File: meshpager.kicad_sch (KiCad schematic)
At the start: 0 parts

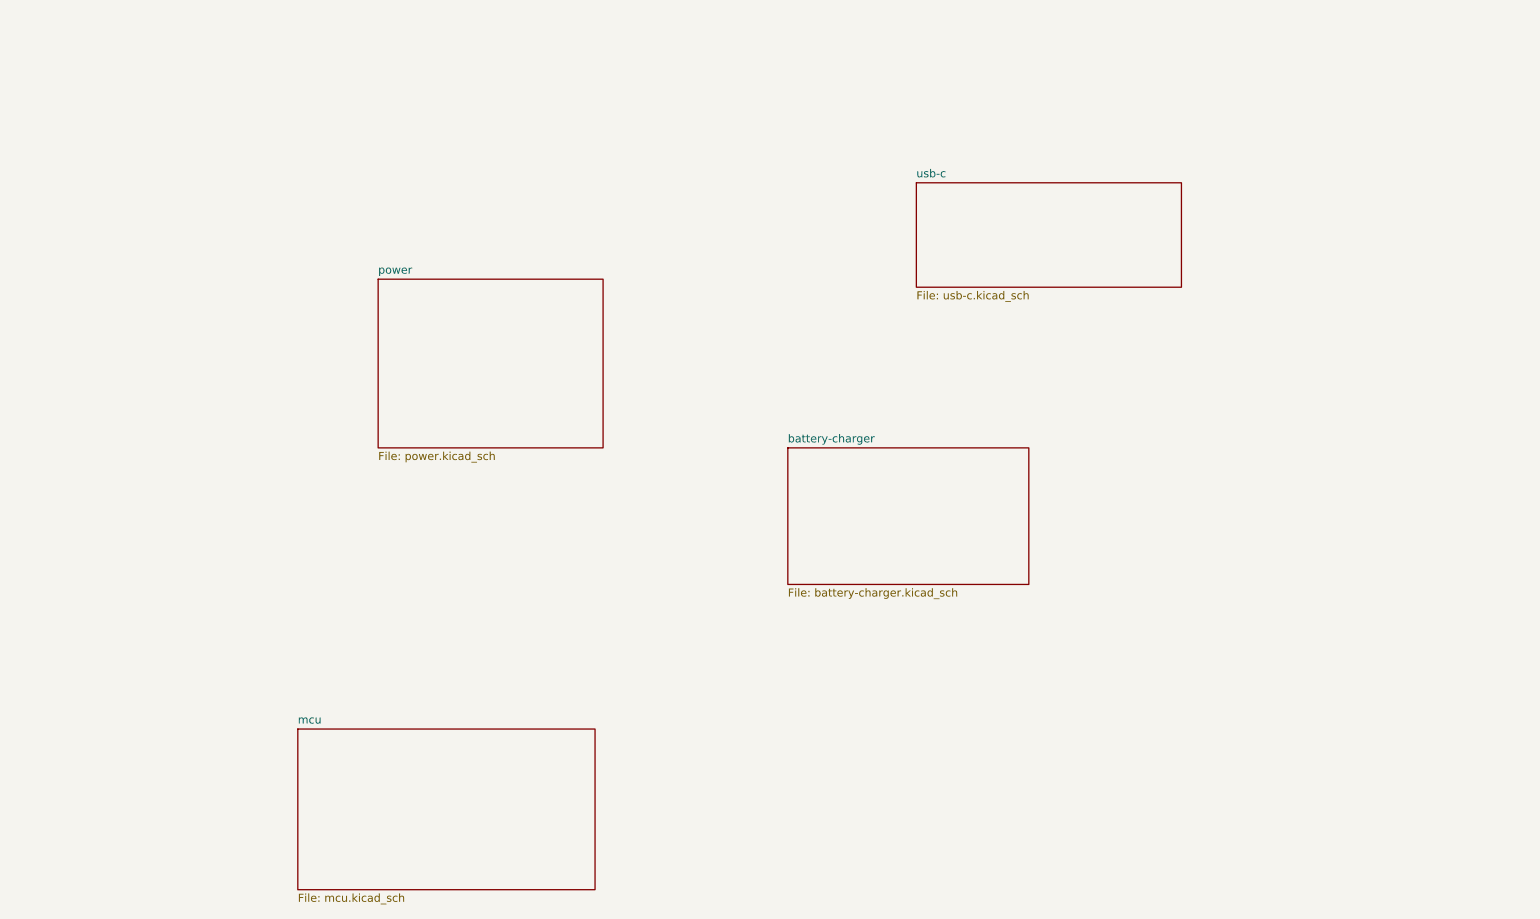
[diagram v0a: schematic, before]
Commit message: update
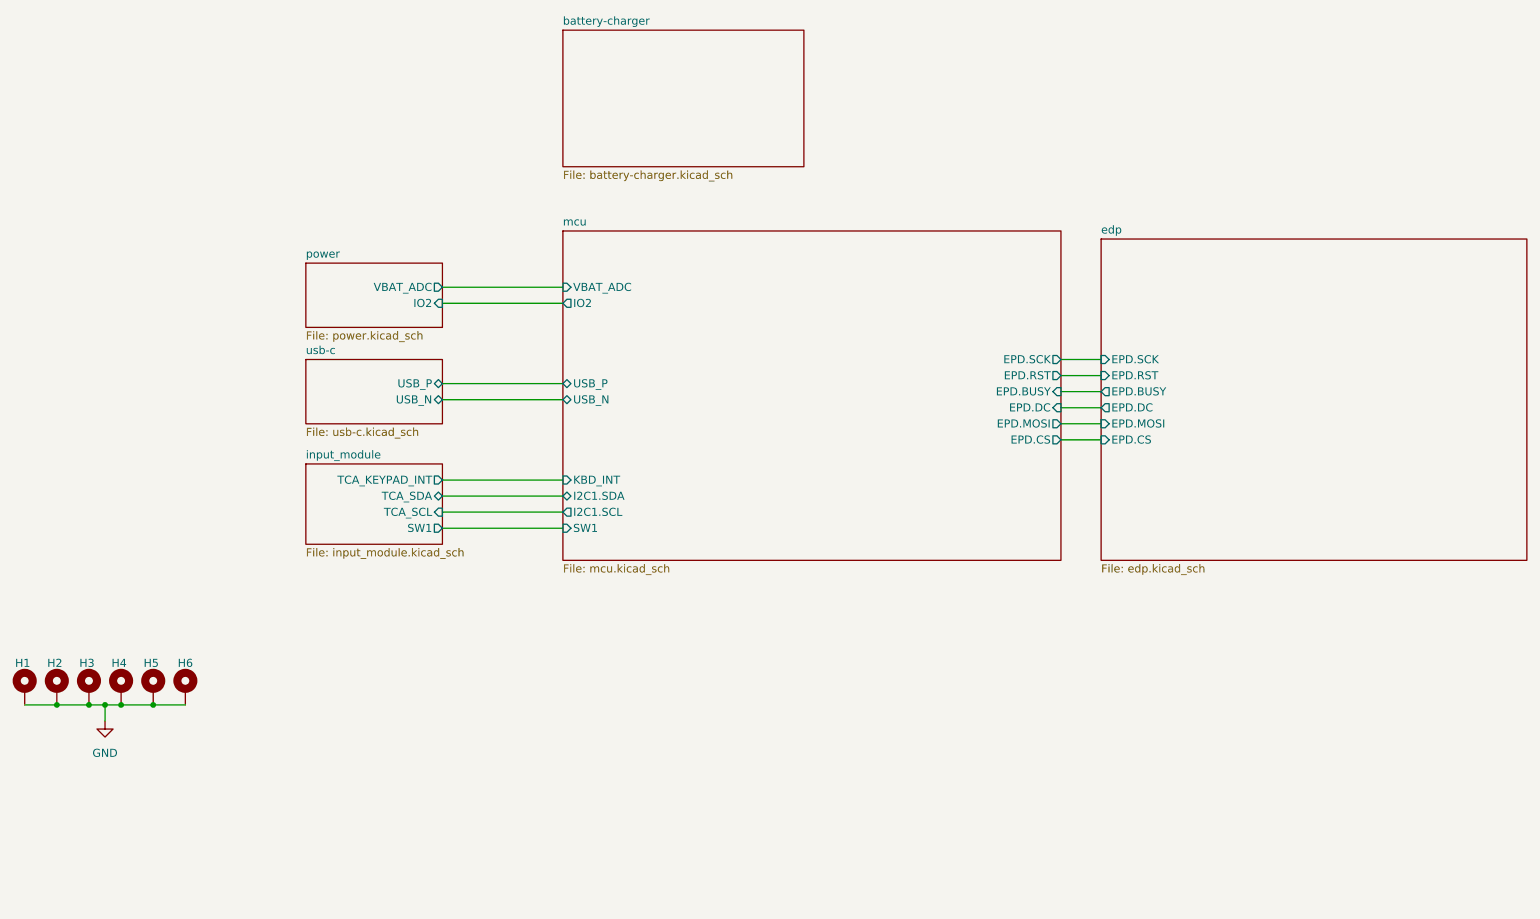
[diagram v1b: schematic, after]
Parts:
- added H1, H2, H3, H4, H5, H6: MountingHole_Pad, MountingHole:MountingHole_2.7mm_M2.5_Pad, symbol Mechanical:MountingHole_Pad
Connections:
- new net GND: H1.1, H2.1, H3.1, H4.1, H5.1, H6.1
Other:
- added sheet edp (edp.kicad_sch)
- added sheet input_module (input_module.kicad_sch)
- sheet mcu ports: added EPD.BUSY, EPD.CS, EPD.DC, EPD.MOSI, EPD.RST, EPD.SCK, I2C1.SCL, I2C1.SDA, IO2, KBD_INT, SW1, USB_N, USB_P, VBAT_ADC; removed none
- sheet power ports: added IO2, VBAT_ADC; removed none
- sheet usb-c ports: added USB_N, USB_P; removed none
